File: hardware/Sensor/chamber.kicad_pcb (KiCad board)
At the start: 2 copper layers, 100 x 100 mm, 60 parts, among them J1 USB_B_Micro, J10 RF_Shield_Two_Pieces, J11 Conn_Coaxial, J20 RF_Shield_Two_Pieces, Q20 BC859, Q21 Q_NMOS_GDS, SW1 SW_DPDT_x2, U10 LMC662, U11 LM358, U20 MC34063AD, U30 STM32F070F6Px, U31 MCP3425A0T-ECH

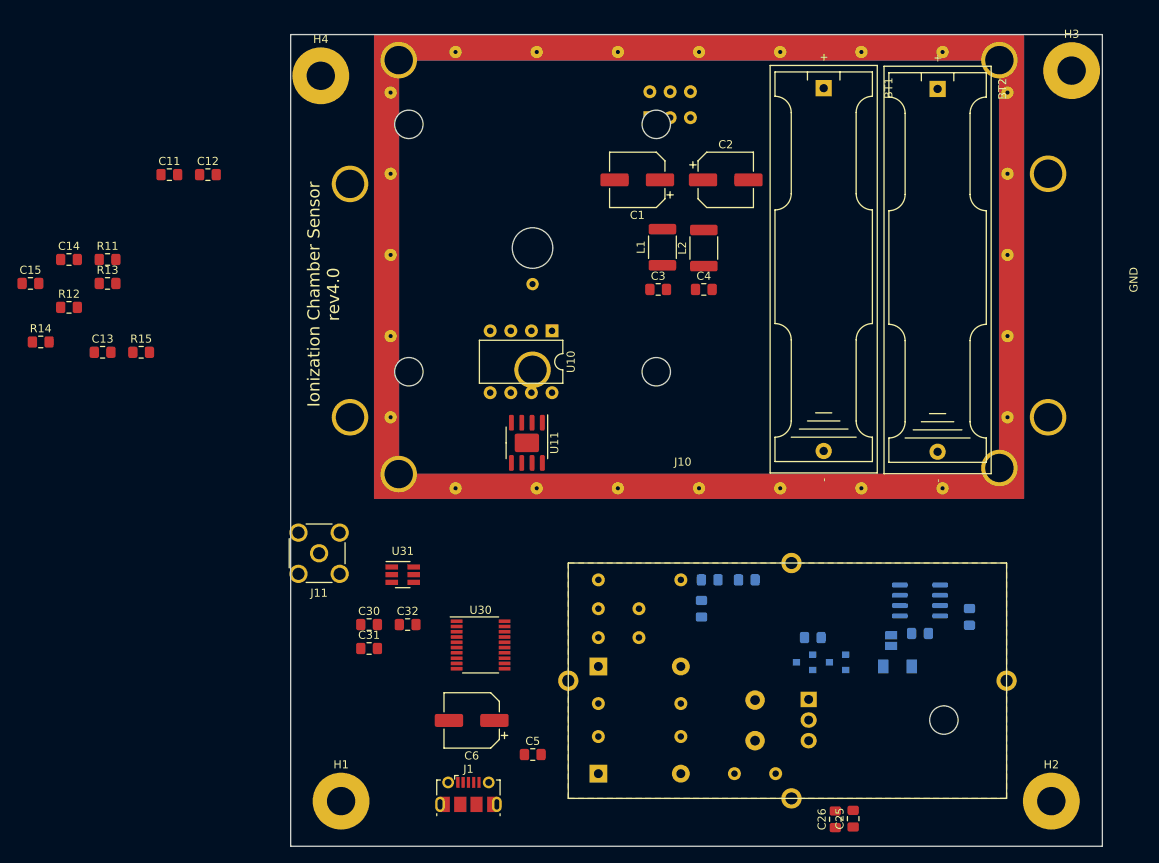
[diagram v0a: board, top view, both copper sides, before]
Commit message: grouped elements and grounds
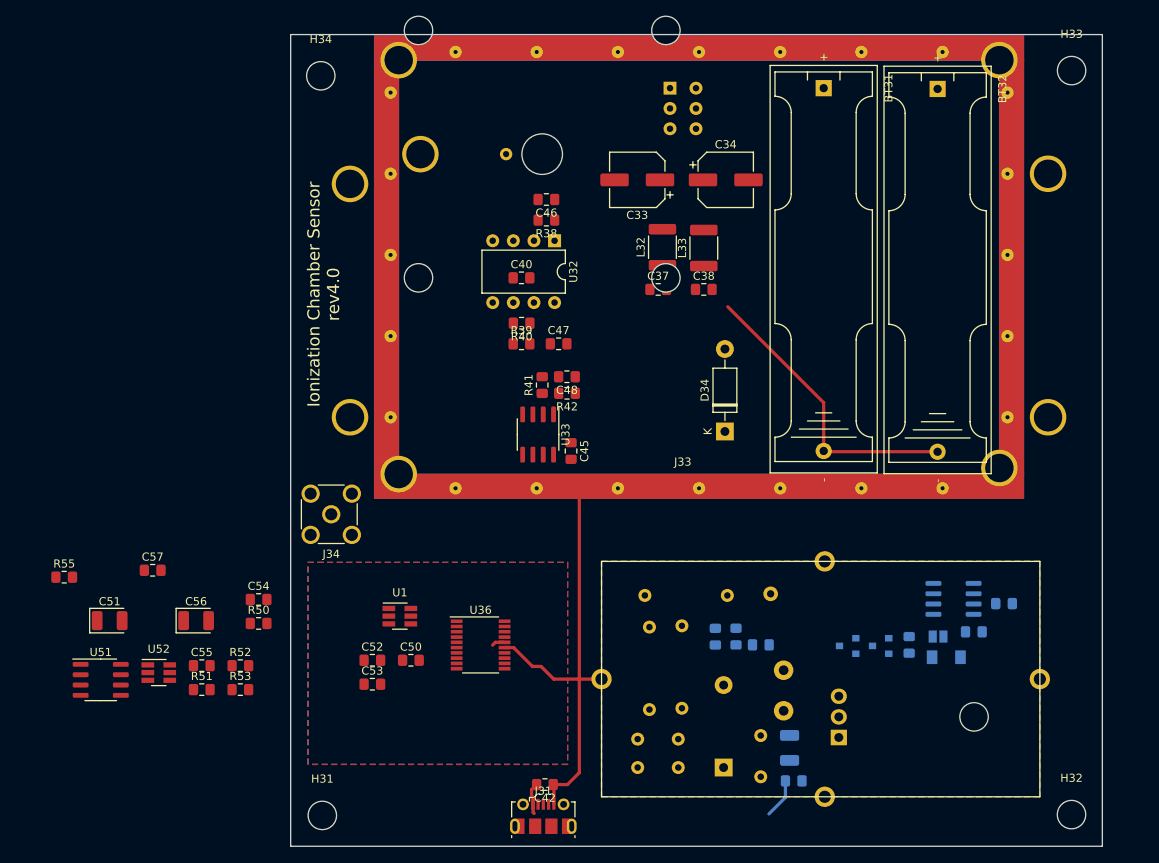
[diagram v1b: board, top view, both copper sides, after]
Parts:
- removed C25, C26, C5: 100n, Capacitor_SMD:C_0805_2012Metric_Pad1.15x1.40mm_HandSolder
- removed D20: 1N4007, Diode_THT:D_DO-41_SOD81_P10.16mm_Horizontal
- removed J10: RF_Shield_Two_Pieces, IonizationChamber:IonizationChamberShield
- added C35: 100n, Capacitor_SMD:C_0805_2012Metric_Pad1.15x1.40mm_HandSolder, B.Cu at (62.0, 91.9)
- added C42: 100n, Capacitor_SMD:C_0805_2012Metric_Pad1.15x1.40mm_HandSolder, F.Cu at (31.3, 92.4)
- added C51: 10n, Capacitor_Tantalum_SMD:CP_EIA-3528-21_Kemet-B, F.Cu at (-22.3, 72.2)
- added C54: 100n, Capacitor_SMD:C_0805_2012Metric_Pad1.15x1.40mm_HandSolder, F.Cu at (-3.95, 69.6)
- added C55: 100n, Capacitor_SMD:C_0805_2012Metric_Pad1.15x1.40mm_HandSolder, F.Cu at (-10.9, 77.8)
- added C56: 10n, Capacitor_Tantalum_SMD:CP_EIA-3528-21_Kemet-B, F.Cu at (-11.7, 72.2)
- added C57: 100n, Capacitor_SMD:C_0805_2012Metric_Pad1.15x1.40mm_HandSolder, F.Cu at (-17.0, 66.0)
- added D33: 1N4007, Diode_THT:D_DO-41_SOD81_P10.16mm_Horizontal, B.Cu at (53.3, 90.3)
- added J33: RF_Shield_Two_Pieces, IonizationChamber:IonizationChamberShield, F.Cu at (10.3, 57.1)
- added R50: 0R, Resistor_SMD:R_0805_2012Metric_Pad1.15x1.40mm_HandSolder, F.Cu at (-3.95, 72.5)
- added R51: 0R, Resistor_SMD:R_0805_2012Metric_Pad1.15x1.40mm_HandSolder, F.Cu at (-10.9, 80.7)
- added R52: 22k, Resistor_SMD:R_0805_2012Metric_Pad1.15x1.40mm_HandSolder, F.Cu at (-6.20, 77.8)
- added R53: R, Resistor_SMD:R_0805_2012Metric_Pad1.15x1.40mm_HandSolder, F.Cu at (-6.20, 80.7)
- added R55: R, Resistor_SMD:R_0805_2012Metric_Pad1.15x1.40mm_HandSolder, F.Cu at (-27.9, 66.8)
- added TP30: TestPoint, TestPoint:TestPoint_Loop_D2.60mm_Drill0.9mm_Beaded, B.Cu at (59.1, 68.9)
- added U51: Opamp_Dual_Generic, Package_SO:SOIC-8_3.9x4.9mm_P1.27mm, F.Cu at (-23.4, 79.5)
- added U52: MCP3425A0T-ECH, Package_TO_SOT_SMD:SOT-23-6_Handsoldering, F.Cu at (-16.2, 78.6)
- C44: renamed from C6; footprint Capacitor_SMD:CP_Elec_6.3x5.4 -> Capacitor_Tantalum_SMD:CP_EIA-3528-21_Kemet-B; moved to B.Cu
- D34: renamed from D22; moved to F.Cu
- H31: renamed from H1; footprint MountingHole:MountingHole_3.5mm_Pad -> MountingHole:MountingHole_3.5mm
- H32: renamed from H2; footprint MountingHole:MountingHole_3.5mm_Pad -> MountingHole:MountingHole_3.5mm
- H33: renamed from H3; footprint MountingHole:MountingHole_3.5mm_Pad -> MountingHole:MountingHole_3.5mm
- H34: renamed from H4; footprint MountingHole:MountingHole_3.5mm_Pad -> MountingHole:MountingHole_3.5mm
- Q32: renamed from Q21; footprint Package_TO_SOT_THT:TO-220-3_Horizontal_TabUp -> Package_TO_SOT_THT:TO-220-3_Horizontal_TabDown
- U33: renamed from U11; footprint Package_SO:SOIC-8-1EP_3.9x4.9mm_P1.27mm_EP2.29x3mm -> Package_SO:SOIC-8_3.9x4.9mm_P1.27mm
- moved C45 69.7 mm to (34.5, 51.3), turned to 270 degrees
- moved R41 62.0 mm to (31.0, 43.2), turned to 90 degrees
- moved C48 57.3 mm to (34.0, 42.2), turned to 180 degrees
- moved R39 55.9 mm to (28.4, 38.1)
- moved C40 55.8 mm to (28.4, 30.0)
- moved R38 54.3 mm to (31.5, 22.9), turned to 180 degrees
- moved R42 52.7 mm to (34.0, 44.2), turned to 180 degrees
- moved R40 51.3 mm to (28.5, 35.6), turned to 180 degrees
- moved C47 48.0 mm to (33.0, 38.1)
- moved C46 46.6 mm to (31.5, 20.3), turned to 180 degrees
- moved D34 44.9 mm to (53.5, 48.9), turned to 90 degrees
- moved C44 39.3 mm to (61.5, 87.9), turned to 90 degrees
- moved R37 23.6 mm to (53.8, 69.1), turned to 180 degrees
- moved C41 21.9 mm to (47.8, 90.3), turned to 180 degrees
- moved R33 18.9 mm to (48.2, 83.0), turned to 90 degrees
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- renumbered BT1 to BT31, BT2 to BT32, C21 to C31, C20 to C32, C1 to C33, C2 to C34, C3 to C37, C4 to C38, C22 to C39, C14 to C40, C23 to C41, C24 to C43, C15 to C45, C11 to C46, C12 to C47, C13 to C48, C32 to C50, C30 to C52, C31 to C53, D23 to D31, D21 to D32, J1 to J31, J20 to J32, J11 to J34, JP20 to JP31, L20 to L31, L1 to L32, L2 to L33, Q20 to Q31, R20 to R31, R21 to R32, R22 to R33, R23 to R34, R24 to R35, R25 to R36, R26 to R37, R11 to R38, R12 to R39, R13 to R40, R14 to R41, R15 to R42, SW1 to SW31, U31 to U1, U20 to U31, U10 to U32, U30 to U36, V10 to V31
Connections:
- C48 pad 1: Net-(C13-Pad1) -> Net-(C48-Pad1)
- C48 pad 2: GND -> Net-(C48-Pad2)
- R40 pad 1: Net-(R13-Pad1) -> Net-(C48-Pad1)
- R41 pad 2: Net-(C13-Pad1) -> Net-(C48-Pad2)
- U32 pad 7: Net-(R13-Pad1) -> Net-(C48-Pad1)
- U33 pad 3: Net-(R13-Pad1) -> GND
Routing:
- net GND: track 0.00 -> 96.4 mm
- net +5V: track 0.00 -> 10.5 mm
- added copper zone on B.Cu, net GND
- removed copper zone on B.Cu, net (none)
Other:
- board text removed: "GND"
